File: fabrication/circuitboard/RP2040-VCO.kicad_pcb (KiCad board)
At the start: 2 copper layers, 29 x 60 mm, 41 parts, among them J2 Power Input, J6 Conn_01x06_Male, J7 Conn_01x08_Male, U1 TL074, U2 Seed_XIAO_RP2040, U3 AP2210K-5.0TRG1

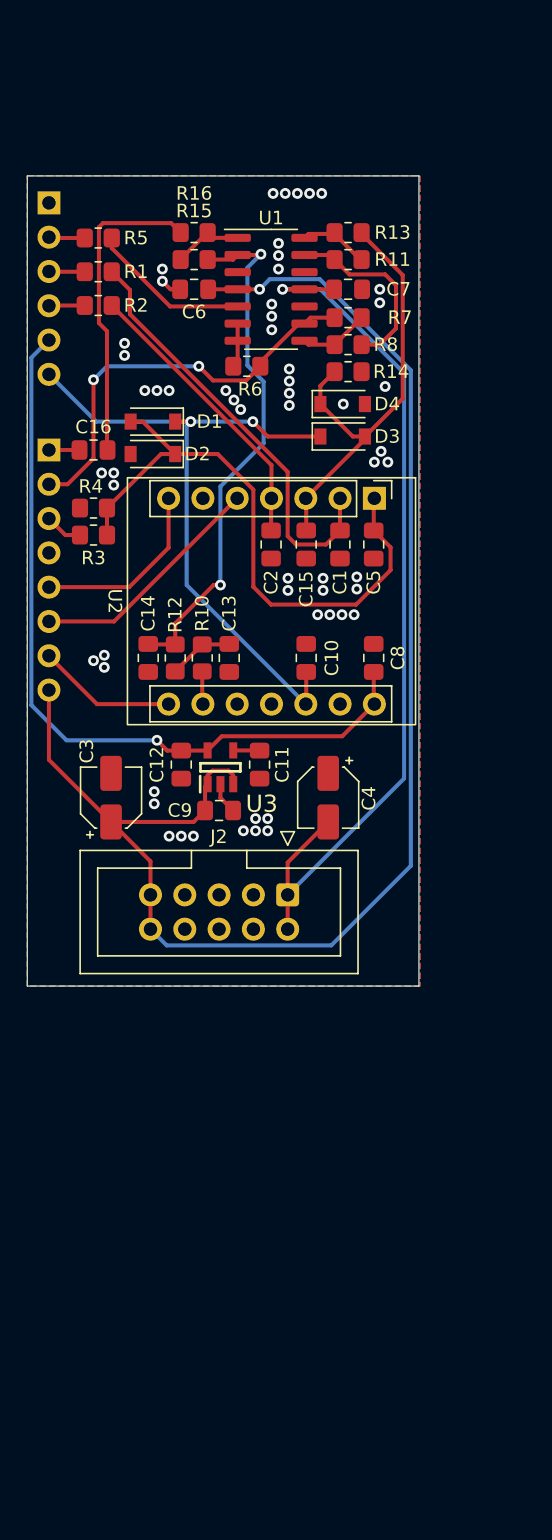
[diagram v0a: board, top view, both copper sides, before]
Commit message: update to v1.1
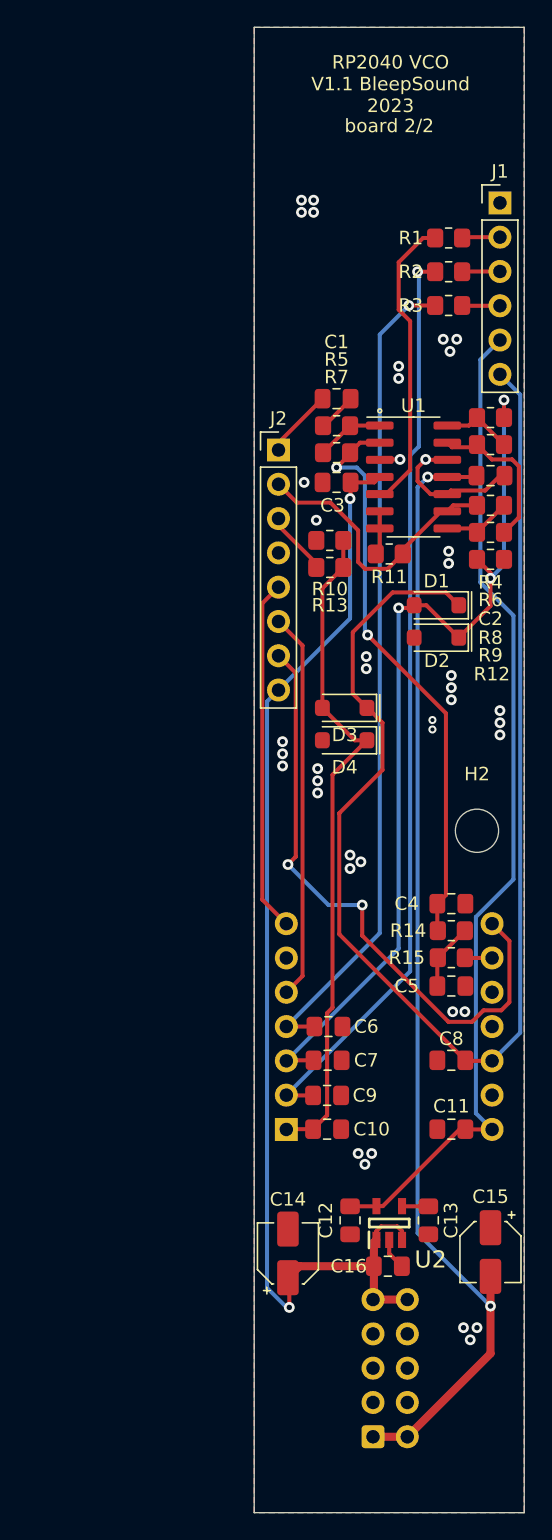
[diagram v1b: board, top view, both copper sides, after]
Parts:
- removed J6: Conn_01x06_Male, Connector_PinHeader_2.54mm:PinHeader_1x06_P2.54mm_Horizontal
- removed J7: Conn_01x08_Male, Connector_PinHeader_2.54mm:PinHeader_1x08_P2.54mm_Horizontal
- added H2: SpacerHoles, MountingHole:MountingHole_3.2mm_M3, F.Cu at (68.0, 96.0)
- added J1: Conn_01x06_Male, Connector_PinHeader_2.54mm:PinHeader_1x06_P2.54mm_Vertical, F.Cu at (69.7, 49.5)
- added J2: Conn_01x08_Male, Connector_PinHeader_2.54mm:PinHeader_1x08_P2.54mm_Vertical, F.Cu at (53.3, 67.8)
- D1: renamed from D3; footprint Diode_SMD:D_SOD-123 -> Kicad-perso:D_SOD-123
- D2: renamed from D4; footprint Diode_SMD:D_SOD-123 -> Kicad-perso:D_SOD-123
- D3: renamed from D1; footprint Diode_SMD:D_SOD-123 -> Kicad-perso:D_SOD-123
- D4: renamed from D2; footprint Diode_SMD:D_SOD-123 -> Kicad-perso:D_SOD-123
- J8: renamed from J2; moved to B.Cu
- U1: footprint Package_SO:SOIC-14_3.9x8.7mm_P1.27mm -> Kicad-perso:SOIC-14_3.9x8.7mm_P1.27mm
- U3: renamed from U2; moved to B.Cu
- moved C10 43.4 mm to (56.9, 118.1), turned to 0 degrees
- moved C9 40.8 mm to (56.9, 115.6), turned to 0 degrees
- moved J8 40.6 mm to (60.3, 140.9), turned to 0 degrees
- moved C7 38.2 mm to (56.9, 113.0), turned to 0 degrees
- moved C14 36.2 mm to (54.0, 127.3)
- moved C13 36.0 mm to (64.4, 124.8)
- moved C12 36.0 mm to (58.6, 124.8)
- moved C16 36.0 mm to (61.4, 128.2)
- moved U2 36.0 mm to (61.5, 125.0)
- moved C6 36.0 mm to (57.0, 110.5), turned to 0 degrees
- moved C15 35.7 mm to (69.0, 127.2)
- moved C11 35.4 mm to (66.1, 118.1), turned to 180 degrees
- moved U3 32.7 mm to (61.5, 110.5), turned to 0 degrees
- moved C8 31.7 mm to (66.1, 113.0), turned to 180 degrees
- moved C5 29.3 mm to (66.1, 107.5), turned to 0 degrees
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- renumbered C16 to C1, C5 to C10, C8 to C11, C11 to C13, C3 to C14, C4 to C15, C9 to C16, C7 to C2, C6 to C3, C14 to C4, C13 to C5, C2 to C6, C15 to C7, C10 to C8, C1 to C9, R5 to R1, R4 to R10, R6 to R11, R14 to R12, R3 to R13, R12 to R14, R10 to R15, R1 to R2, R2 to R3, R13 to R4, R16 to R5, R11 to R6, R15 to R7, R7 to R8, R8 to R9, U3 to U2
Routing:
- net +3V3: track 50.3 -> 101.6 mm, vias 2 -> 0
- net /Chord: track 21.6 -> 61.2 mm, vias 0 -> 1
- net /Tune: track 31.9 -> 68.4 mm, vias 0 -> 1
- net /SW_1: track 10.3 -> 45.7 mm, vias 0 -> 2
- net /Inv: track 33.3 -> 66.9 mm, vias 0 -> 3
- net +12V: track 110.7 -> 86.3 mm, vias 1 -> 2
- net Net-(C1-Pad2): track 23.2 -> 2.90 mm
- net -12V: track 66.8 -> 84.5 mm, vias 1 -> 2
- net +5V: track 58.2 -> 74.6 mm, vias 1 -> 0
- net /SW_0: track 13.7 -> 26.2 mm
- net /Push_SW: track 17.7 -> 28.7 mm
- net GND: track 3.90 -> 14.7 mm, vias 58 -> 42
- net Net-(U1B-+): track 11.9 -> 22.2 mm
- net /InvJack: track 30.7 -> 20.8 mm, vias 2 -> 0
- net /V/oct: track 44.7 -> 49.8 mm
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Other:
- board size 29 x 60 mm -> 20 x 110 mm
- board text added: "RP2040 VCO V1.1 BleepSound 2023"
- board text removed: "RP2040 VCO V1.0 BleepSound 2023"
